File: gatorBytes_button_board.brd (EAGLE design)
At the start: 100.3 x 54.6 mm, 45 parts

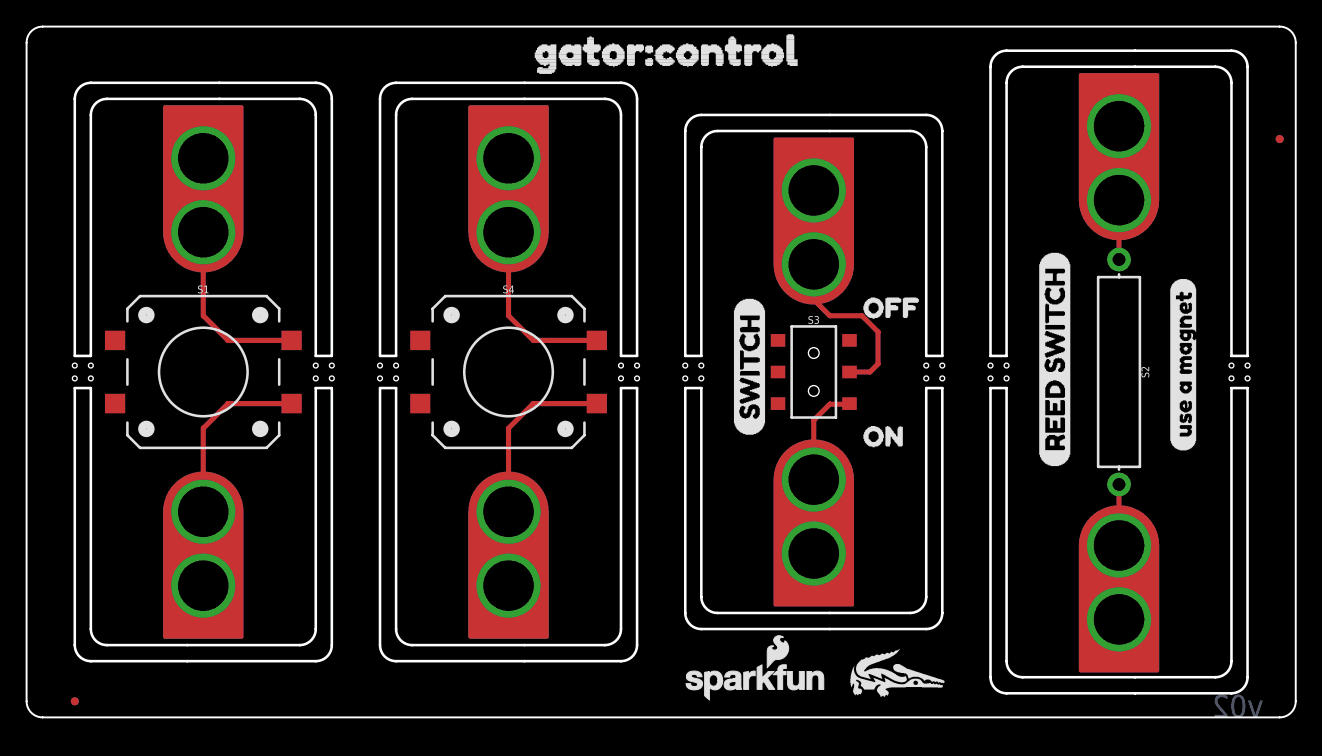
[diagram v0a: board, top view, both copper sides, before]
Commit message: post checklist changes
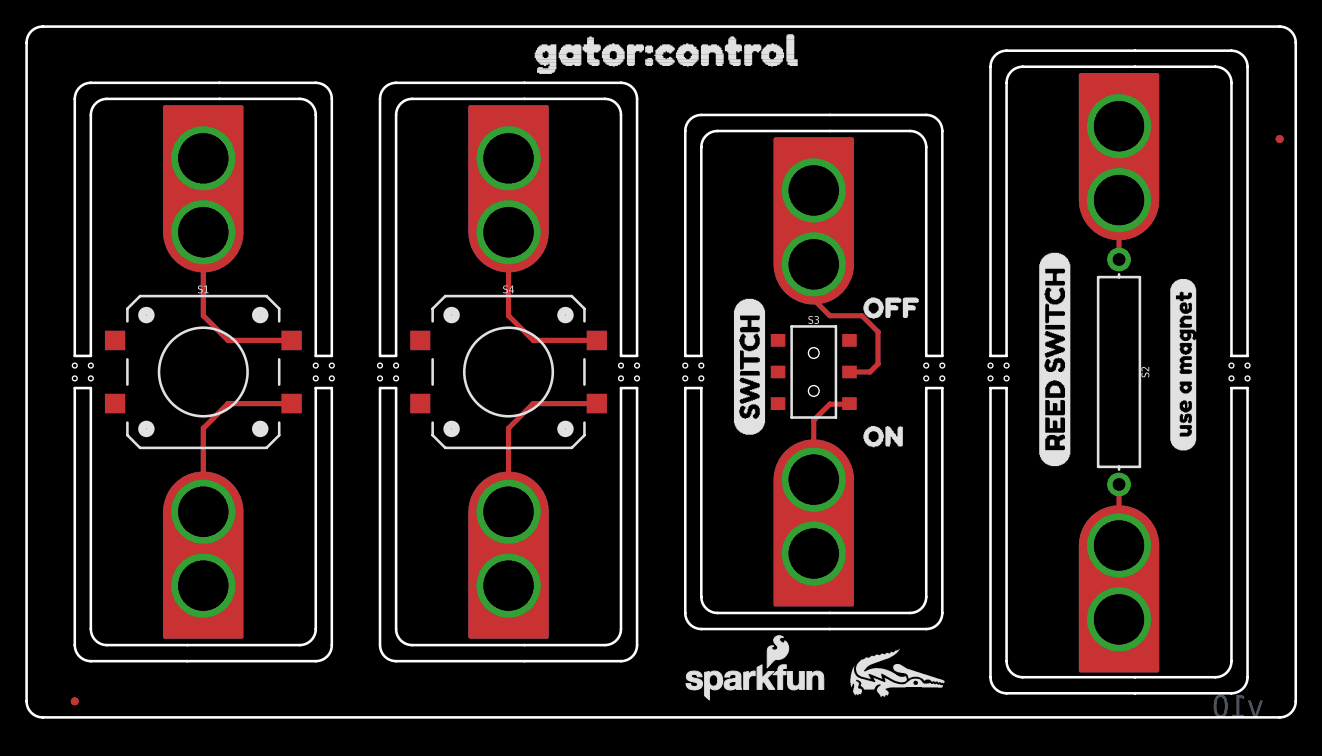
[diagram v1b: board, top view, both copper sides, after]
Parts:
- moved LOGO6 5.08 mm to (8.13, 45.1)
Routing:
- net N$7: track 17.7 -> 26.8 mm
- net N$4: track 14.4 -> 20.5 mm
- net N$2: track 15.8 -> 21.9 mm
- net N$1: track 14.4 -> 20.2 mm
- net N$3: track 14.4 -> 20.2 mm
- net N$9: track 13.9 -> 15.9 mm
- net N$6: track 10.7 -> 12.3 mm
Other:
- board text added: "v10"
- board text removed: "v02"
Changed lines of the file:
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@@
 <hole x="77.47" y="26.797" drill="0.381"/>
 <hole x="77.47" y="27.813" drill="0.381"/>
-<wire x1="1.27" y1="0" x2="0" y2="1.27" width="0.1524" layer="20" curve="-90"/>
-<wire x1="0" y1="1.27" x2="0" y2="53.34" width="0.1524" layer="20"/>
-<wire x1="0" y1="53.34" x2="1.27" y2="54.61" width="0.1524" layer="20" curve="-90"/>
-<wire x1="1.27" y1="54.61" x2="99.06" y2="54.61" width="0.1524" layer="20"/>
-<wire x1="99.06" y1="54.61" x2="100.33" y2="53.34" width="0.1524" layer="20" curve="-90"/>
-<wire x1="100.33" y1="53.34" x2="100.33" y2="1.27" width="0.1524" layer="20"/>
-<wire x1="100.33" y1="1.27" x2="99.06" y2="0" width="0.1524" layer="20" curve="-90"/>
-<wire x1="99.06" y1="0" x2="1.27" y2="0" width="0.1524" layer="20"/>
-<text x="97.79" y="0" size="1.778" layer="16" font="vector" ratio="15" rot="MR0">v02</text>
+<wire x1="1.27" y1="0" x2="0" y2="1.27" width="0.2032" layer="20" curve="-90"/>
+<wire x1="0" y1="1.27" x2="0" y2="53.34" width="0.2032" layer="20"/>
+<wire x1="0" y1="53.34" x2="1.27" y2="54.61" width="0.2032" layer="20" curve="-90"/>
+<wire x1="1.27" y1="54.61" x2="99.06" y2="54.61" width="0.2032" layer="20"/>
+<wire x1="99.06" y1="54.61" x2="100.33" y2="53.34" width="0.2032" layer="20" curve="-90"/>
+<wire x1="100.33" y1="53.34" x2="100.33" y2="1.27" width="0.2032" layer="20"/>
+<wire x1="100.33" y1="1.27" x2="99.06" y2="0" width="0.2032" layer="20" curve="-90"/>
+<wire x1="99.06" y1="0" x2="1.27" y2="0" width="0.2032" layer="20"/>
+<text x="97.79" y="0" size="1.778" layer="16" font="vector" ratio="15" rot="MR0">v10</text>
 <text x="49.53" y="-9.525" size="1.778" layer="51" font="vector" ratio="15">M. West</text>
 <text x="6.4135" y="4.7625" size="0.8128" layer="51" font="vector" ratio="15">route out</text>
@@
 <element name="LOGO4" library="SparkFun-Aesthetics" library_urn="urn:adsk.eagle:library:507" package="SFE_LOGO_FLAME_.1" package3d_urn="urn:adsk.eagle:package:37114/1" value="SFE_LOGO_FLAME.1_INCH" x="32.385" y="45.085" rot="MR0"/>
 <element name="LOGO5" library="SparkFun-Aesthetics" library_urn="urn:adsk.eagle:library:507" package="OSHW-LOGO-S" package3d_urn="urn:adsk.eagle:package:37099/1" value="OSHW-LOGOS" x="20.193" y="46.355" rot="MR0"/>
-<element name="LOGO6" library="SparkFun-Aesthetics" library_urn="urn:adsk.eagle:library:507" package="SFE_LOGO_FLAME_.1" package3d_urn="urn:adsk.eagle:package:37114/1" value="SFE_LOGO_FLAME.1_INCH" x="8.128" y="40.005" rot="MR0"/>
+<element name="LOGO6" library="SparkFun-Aesthetics" library_urn="urn:adsk.eagle:library:507" package="SFE_LOGO_FLAME_.1" package3d_urn="urn:adsk.eagle:package:37114/1" value="SFE_LOGO_FLAME.1_INCH" x="8.128" y="45.085" rot="MR0"/>
 <element name="U$33" library="SparkFun-Aesthetics" package="ORDERING_INSTRUCTIONS" value="" x="-3.81" y="-12.065"/>
 <element name="S1" library="SparkFun-Switches" package="TACTILE_SWITCH_SMD_12MM" value="MOMENTARY-SWITCH-SPST-SMD-12MM" x="13.97" y="27.305">
@@
 <wire x1="38.1" y1="22.86" x2="40.045" y2="24.805" width="0.4064" layer="1"/>
 <wire x1="40.045" y1="24.805" x2="45.075" y2="24.805" width="0.4064" layer="1"/>
-<wire x1="38.1" y1="10.414" x2="38.1" y2="16.256" width="0" layer="19" extent="1-1"/>
+<wire x1="38.1" y1="16.256" x2="38.1" y2="10.414" width="0.2032" layer="1"/>
 </signal>
 <signal name="N$2">
@@
 <wire x1="45.075" y1="29.805" x2="40.045" y2="29.805" width="0.4064" layer="1"/>
 <wire x1="40.045" y1="29.805" x2="38.1" y2="31.75" width="0.4064" layer="1"/>
-<wire x1="38.1" y1="31.75" x2="38.1" y2="38.354" width="0.4064" layer="1"/>
-<wire x1="38.1" y1="38.354" x2="38.1" y2="42.7675" width="0" layer="19" extent="1-1"/>
+<wire x1="38.1" y1="31.75" x2="38.1" y2="38.1" width="0.4064" layer="1"/>
+<wire x1="38.1" y1="44.196" x2="38.1" y2="38.1" width="0.2032" layer="1"/>
+<wire x1="38.1" y1="38.354" x2="38.1" y2="38.1" width="0.2032" layer="1"/>
 </signal>
 <signal name="N$3">
@@
 <wire x1="15.915" y1="24.805" x2="13.97" y2="22.86" width="0.4064" layer="1"/>
 <wire x1="13.97" y1="22.86" x2="13.97" y2="16.256" width="0.4064" layer="1"/>
-<wire x1="13.97" y1="10.414" x2="13.97" y2="16.256" width="0" layer="19" extent="1-1"/>
+<wire x1="13.97" y1="16.256" x2="13.97" y2="10.414" width="0.2032" layer="1"/>
 </signal>
 <signal name="N$4">
@@
 <wire x1="20.945" y1="29.805" x2="15.915" y2="29.805" width="0.4064" layer="1"/>
 <wire x1="15.915" y1="29.805" x2="13.97" y2="31.75" width="0.4064" layer="1"/>
-<wire x1="13.97" y1="31.75" x2="13.97" y2="38.354" width="0.4064" layer="1"/>
-<wire x1="13.97" y1="38.354" x2="13.97" y2="44.196" width="0" layer="19" extent="1-1"/>
+<wire x1="13.97" y1="31.75" x2="13.97" y2="38.1" width="0.4064" layer="1"/>
+<wire x1="13.97" y1="44.196" x2="13.97" y2="38.1" width="0.2032" layer="1"/>
+<wire x1="13.97" y1="38.354" x2="13.97" y2="38.1" width="0.2032" layer="1"/>
 </signal>
 <signal name="N$5">
@@
 <wire x1="86.36" y1="40.64" x2="86.36" y2="46.736" width="0.4064" layer="1"/>
 <wire x1="86.36" y1="36.195" x2="86.36" y2="40.64" width="0.4064" layer="1"/>
-<wire x1="86.36" y1="40.64" x2="86.36" y2="40.894" width="0" layer="19" extent="1-1"/>
+<wire x1="86.36" y1="40.894" x2="86.36" y2="40.64" width="0.2032" layer="1"/>
 </signal>
 <signal name="N$6">
@@
 <contactref element="U$12" pad="P$1"/>
 <contactref element="U$12" pad="P$2"/>
-<wire x1="86.36" y1="18.415" x2="86.36" y2="7.747" width="0.4064" layer="1"/>
-<wire x1="86.36" y1="18.415" x2="86.36" y2="13.589" width="0" layer="19" extent="1-1"/>
+<wire x1="86.36" y1="18.415" x2="86.36" y2="15.24" width="0.4064" layer="1"/>
+<wire x1="86.36" y1="15.24" x2="86.36" y2="7.747" width="0.4064" layer="1"/>
+<wire x1="86.36" y1="13.589" x2="86.36" y2="15.24" width="0.4064" layer="1"/>
 </signal>
 <signal name="N$7">
 <contactref element="S3" pad="2"/>
 <contactref element="U$15" pad="P$1"/>
-<wire x1="63.5" y1="38.735" x2="62.1115875" y2="38.735" width="0.4064" layer="1"/>
 <wire x1="60.96" y1="38.735" x2="61.976" y2="38.735" width="0.4064" layer="1"/>
 <contactref element="U$15" pad="P$2"/>
-<wire x1="62.1115875" y1="42.816178125" x2="62.226775" y2="42.7031375" width="0.4064" layer="1"/>
 <wire x1="62.103" y1="38.735" x2="61.976" y2="38.735" width="0.4064" layer="1"/>
-<wire x1="62.228925" y1="41.656" x2="62.226775" y2="42.7031375" width="0.4064" layer="1"/>
 <wire x1="62.1115875" y1="38.735" x2="62.103" y2="38.735" width="0.4064" layer="1"/>
 <wire x1="65.055" y1="27.305" x2="66.675" y2="27.305" width="0.4064" layer="1"/>
@@
 <wire x1="63.5" y1="31.75" x2="62.23" y2="33.02" width="0.4064" layer="1"/>
 <wire x1="62.23" y1="33.02" x2="62.23" y2="35.814" width="0.4064" layer="1"/>
-<wire x1="62.228925" y1="41.656" x2="62.23" y2="41.656" width="0" layer="19" extent="1-1"/>
-<wire x1="62.1115875" y1="38.735" x2="62.23" y2="41.656" width="0" layer="19" extent="1-1"/>
-<wire x1="62.23" y1="35.814" x2="62.1115875" y2="38.735" width="0" layer="19" extent="1-1"/>
+<wire x1="62.23" y1="41.656" x2="62.23" y2="33.02" width="0.2032" layer="1"/>
+<wire x1="62.23" y1="41.656" x2="62.23" y2="38.989" width="0.2032" layer="1"/>
+<wire x1="62.23" y1="38.989" x2="61.976" y2="38.735" width="0.2032" layer="1"/>
 </signal>
 <signal name="N$8">
@@
 <wire x1="63.5" y1="24.765" x2="62.23" y2="23.495" width="0.4064" layer="1"/>
 <contactref element="U$14" pad="P$2"/>
-<wire x1="62.23" y1="23.495" x2="62.23" y2="12.954003125" width="0.4064" layer="1"/>
-<wire x1="62.23" y1="23.495" x2="62.23" y2="18.796" width="0" layer="19" extent="1-1"/>
-<wire x1="62.23" y1="12.954" x2="62.23" y2="12.954003125" width="0" layer="19" extent="1-1"/>
+<wire x1="62.23" y1="23.495" x2="62.23" y2="17.78" width="0.4064" layer="1"/>
+<wire x1="62.23" y1="18.796" x2="62.23" y2="17.78" width="0.4064" layer="1"/>
+<wire x1="62.23" y1="18.796" x2="62.23" y2="12.954" width="0.4064" layer="1"/>
 </signal>
 </signals>
